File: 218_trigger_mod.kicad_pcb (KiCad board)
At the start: 2 copper layers, 52.6 x 44.5 mm, 28 parts, among them J1 Conn_01x06_Female, U1 TL074, U2 TL071

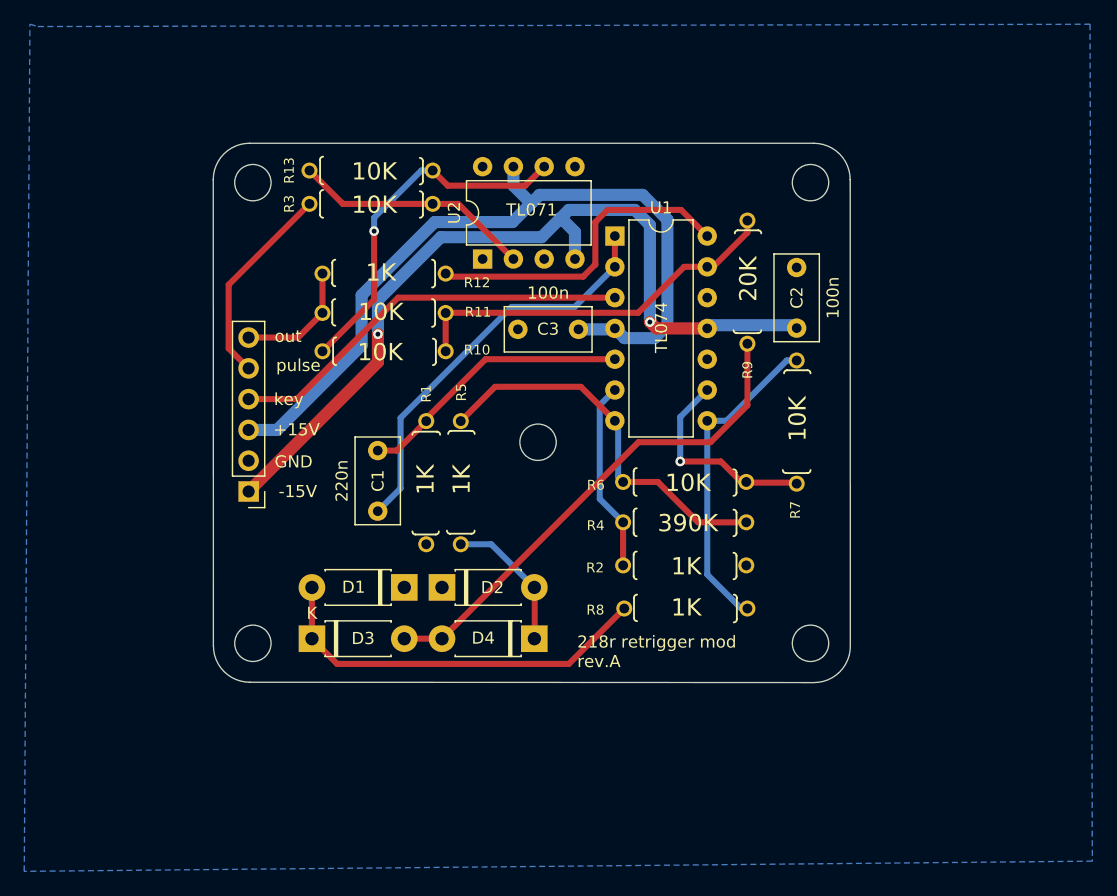
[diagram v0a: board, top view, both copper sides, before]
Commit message: gitignore
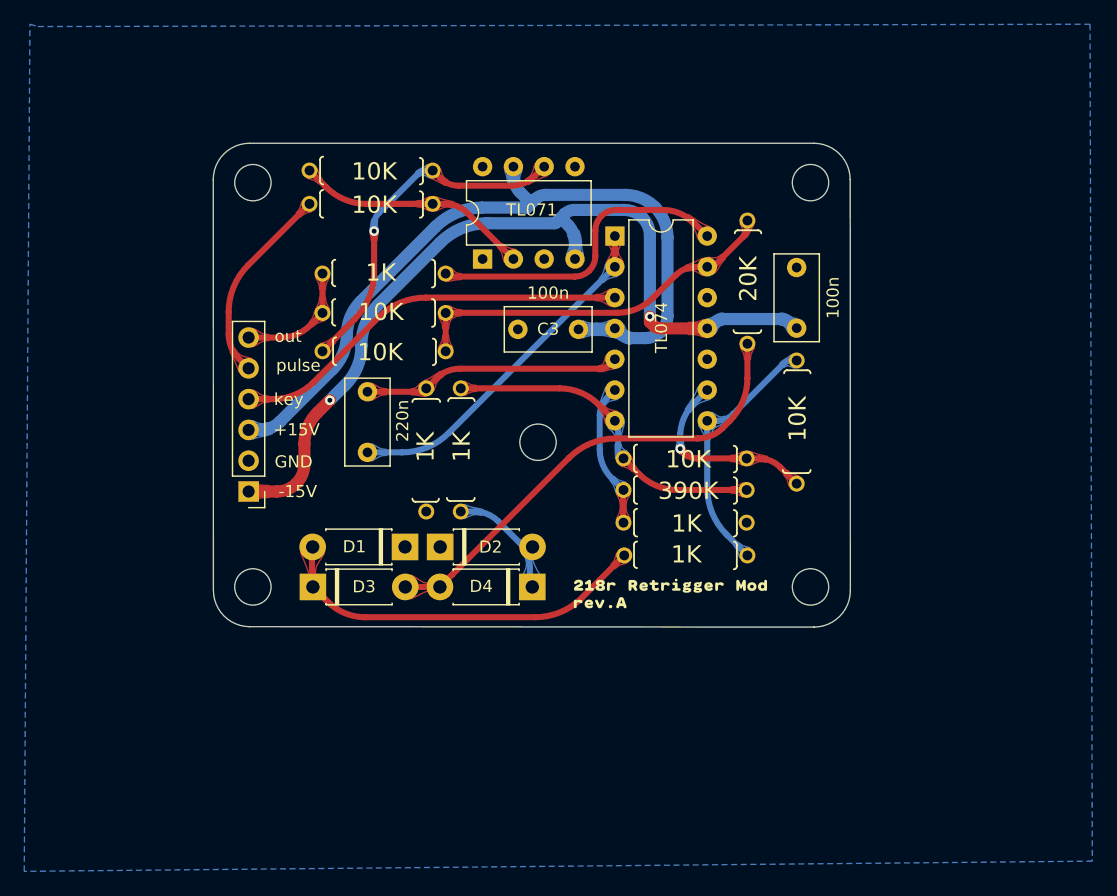
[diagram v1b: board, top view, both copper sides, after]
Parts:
- added kibuzzard-62811A1C: G***, kibuzzard-62811A1C, F.Cu at (155.2, 117.5)
- added kibuzzard-62811A51: G***, kibuzzard-62811A51, F.Cu at (149.4, 118.9)
- moved C1 4.92 mm to (130.2, 106.5)
- moved REF** 4.65 mm to (166.8, 117.6)
- moved REF** 4.65 mm to (120.8, 117.6)
- moved R8 4.38 mm to (156.5, 115.0)
- moved D4 4.27 mm to (143.8, 117.6)
- moved D3 4.27 mm to (125.7, 117.6)
- moved R2 3.52 mm to (156.4, 112.3)
- moved D2 3.34 mm to (136.2, 114.3)
- moved D1 3.34 mm to (133.3, 114.3)
- moved R1 2.70 mm to (135.1, 106.3)
- moved R5 2.70 mm to (137.9, 106.3)
- moved R4 2.67 mm to (156.4, 109.6)
- moved R6 1.94 mm to (156.4, 107.0)
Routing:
- net Net-(R7-Pad2): track 26.6 -> 20.7 mm
- net Net-(C1-Pad1): track 33.9 -> 29.0 mm
- net Net-(R4-Pad2): track 31.5 -> 27.3 mm
- net Net-(R2-Pad1): track 15.8 -> 11.9 mm
- net Net-(D3-Pad2): track 41.7 -> 38.6 mm
- net Net-(D2-Pad2): track 11.2 -> 9.22 mm
- net Net-(C1-Pad2): track 22.6 -> 20.9 mm
- net Net-(D1-Pad2): track 32.8 -> 31.4 mm
- net -15V: track 70.7 -> 71.8 mm
- net Net-(R13-Pad1): track 19.8 -> 18.9 mm
- net +15V: track 66.2 -> 65.2 mm
- net Net-(R10-Pad1): track 29.6 -> 29.0 mm
- net Net-(R12-Pad1): track 26.5 -> 26.0 mm
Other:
- board size 52.6 x 44.5 mm -> 52.6 x 39.9 mm
- board text removed: "218r retrigger mod rev.A"
